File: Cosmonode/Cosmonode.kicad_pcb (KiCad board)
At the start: 2 copper layers, 59.7 x 36.2 mm, 49 parts, among them J1 CONN_01X12, J10 WEEE_Logo, J11 Aloes_Logo, J12 Aloes_mini_Logo, J13 CONN_01X05, J14 GS2, J2 CONN_01X12, J3 GS2, J4 OSHW, J5 CONN_01X02, J6 GS2, J8 USB_OTG, J9 GS2, P1 COAX, SW1 SW_DIP_x01, U1 ATMEGA328P-AU, U2 RFM69CW, U3 RN2483, U5 XC6206P332MR, U6 ATSHA204, U7 MCP73811T-420I/OT, Y1 Crystal_GND2

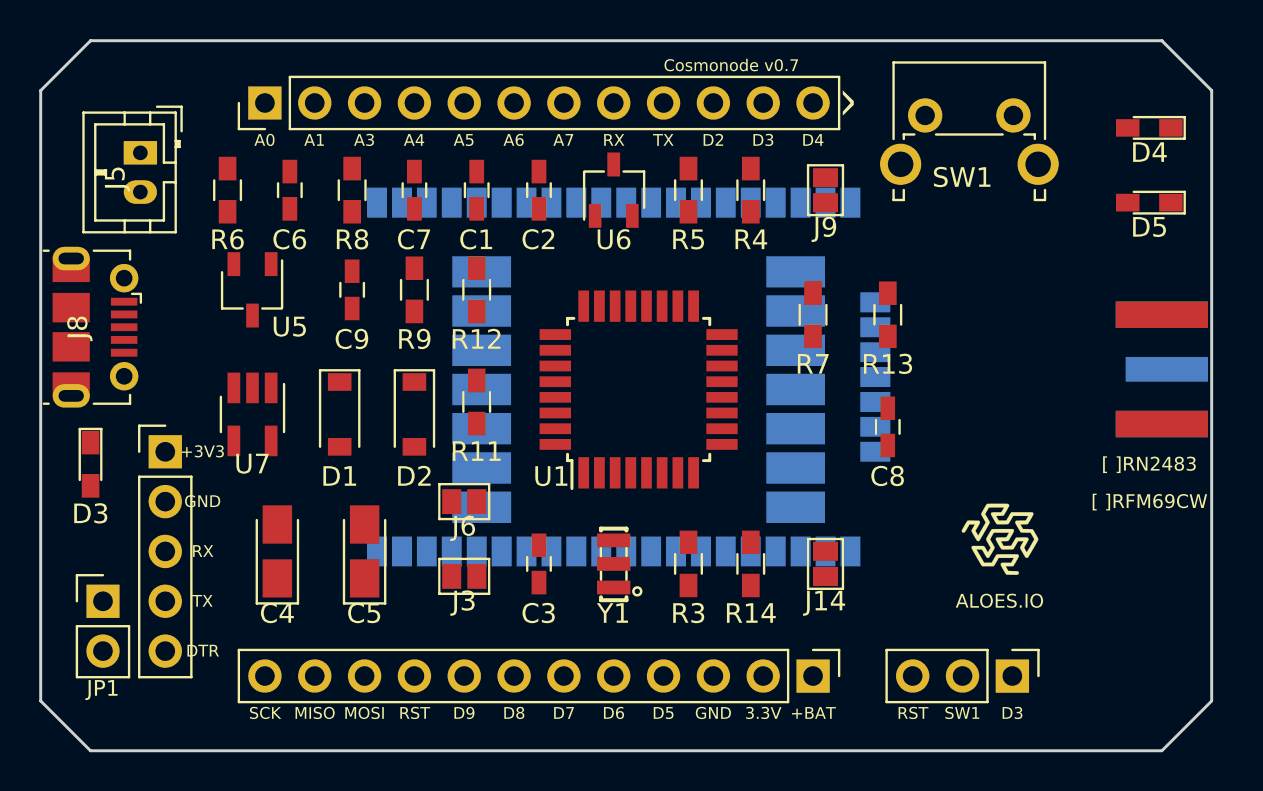
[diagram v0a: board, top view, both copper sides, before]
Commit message: start v0.8
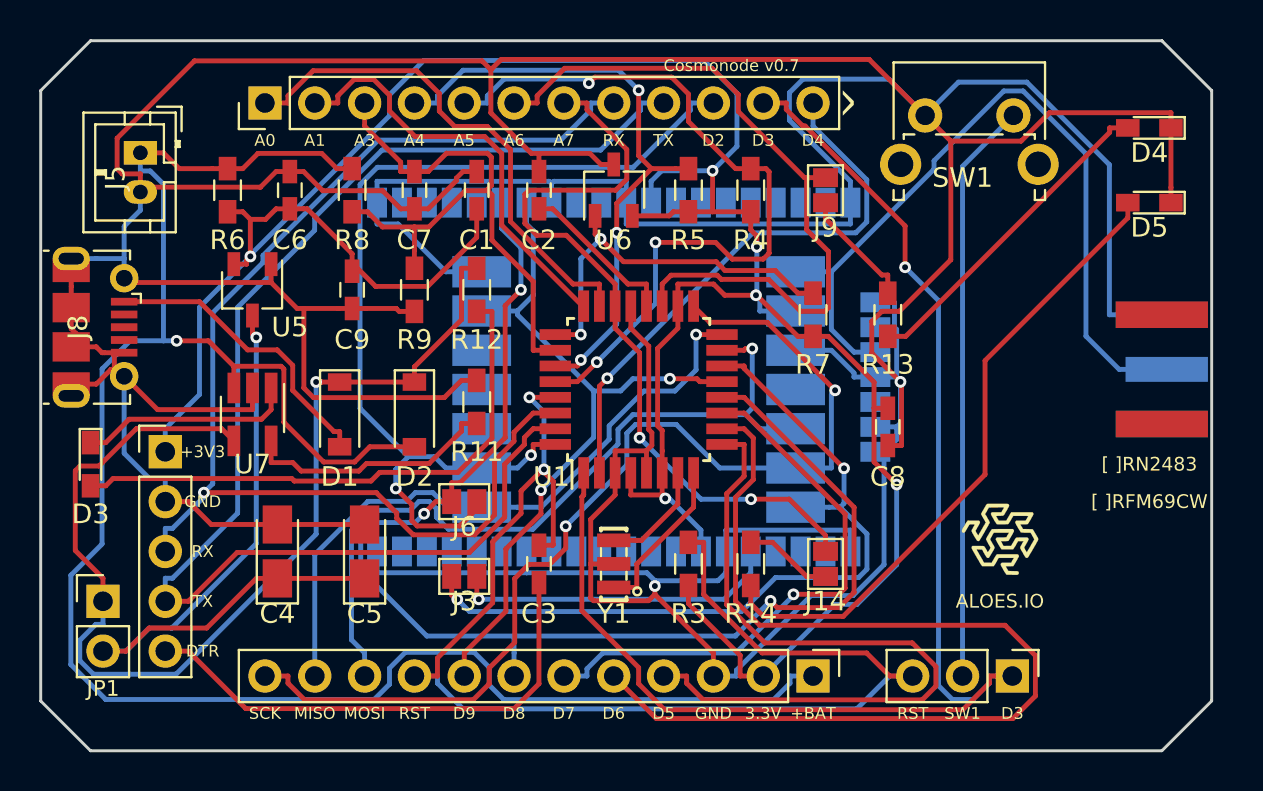
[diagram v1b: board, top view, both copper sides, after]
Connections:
- P1 pad 3: (no net) -> GND
- P1 pad 4: (no net) -> GND
- P1 pad 5: (no net) -> GND
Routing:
- net GND: track 0.00 -> 358.8 mm, vias 0 -> 2
- net +3V3: track 0.00 -> 143.6 mm, vias 0 -> 6
- net +BATT: track 0.00 -> 102.2 mm, vias 0 -> 1
- net D3: track 0.00 -> 71.4 mm, vias 0 -> 1
- net TX: track 0.00 -> 68.7 mm
- net D8: track 0.00 -> 67.7 mm, vias 0 -> 3
- net RST: track 0.00 -> 66.8 mm, vias 0 -> 2
- net RX: track 0.00 -> 62.1 mm, vias 0 -> 1
- net Net-(D1-Pad1): track 0.00 -> 55.8 mm, vias 0 -> 1
- net D13/SCK: track 0.00 -> 53.3 mm, vias 0 -> 2
- net D6: track 0.00 -> 51.8 mm
- net D2: track 0.00 -> 51.3 mm, vias 0 -> 2
- net D11/MOSI: track 0.00 -> 40.0 mm, vias 0 -> 1
- net ANT: track 0.00 -> 40.0 mm
- net D10: track 0.00 -> 39.9 mm, vias 0 -> 2
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- added copper zone on B.Cu, net GND
- added copper zone on F.Cu, net GND
